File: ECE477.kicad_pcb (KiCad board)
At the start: 2 copper layers, 88.9 x 88.9 mm, 52 parts, among them IC1 LP3852EMP-3.3_NOPB, IC2 BQ29330DBT, J1 P7805-2000-S, J2 Conn_01x05_Male, J3 Conn_01x05_Male, J4 Conn_01x05_Male, J5 Conn_01x05_Male, J6 Conn_01x05_Male, J7 Conn_01x05_Male, J8 Conn_01x05_Male, SW1 SW_Push_Dual, U1 STM32H7_LQFP144_T2

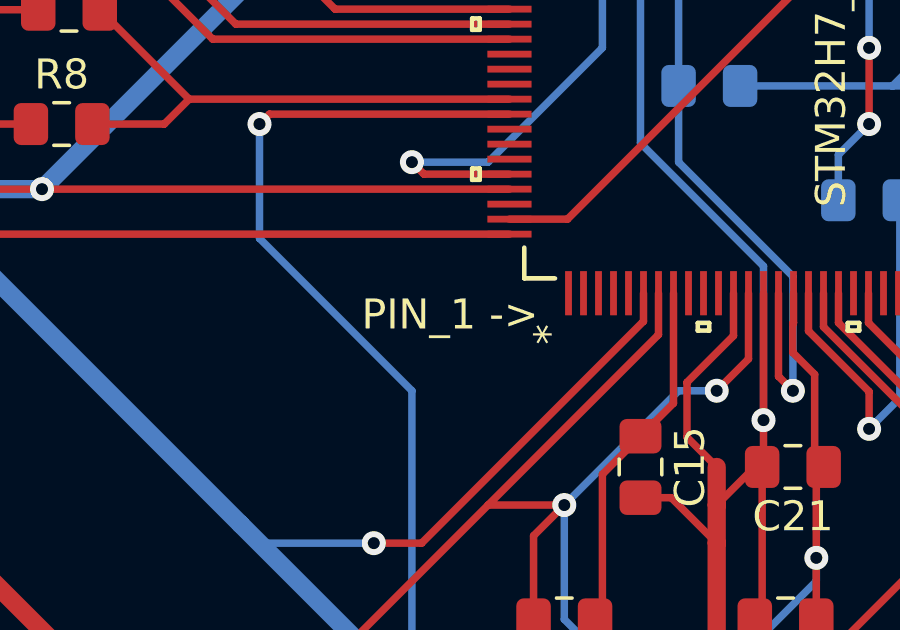
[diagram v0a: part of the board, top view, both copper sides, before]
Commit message: Updated
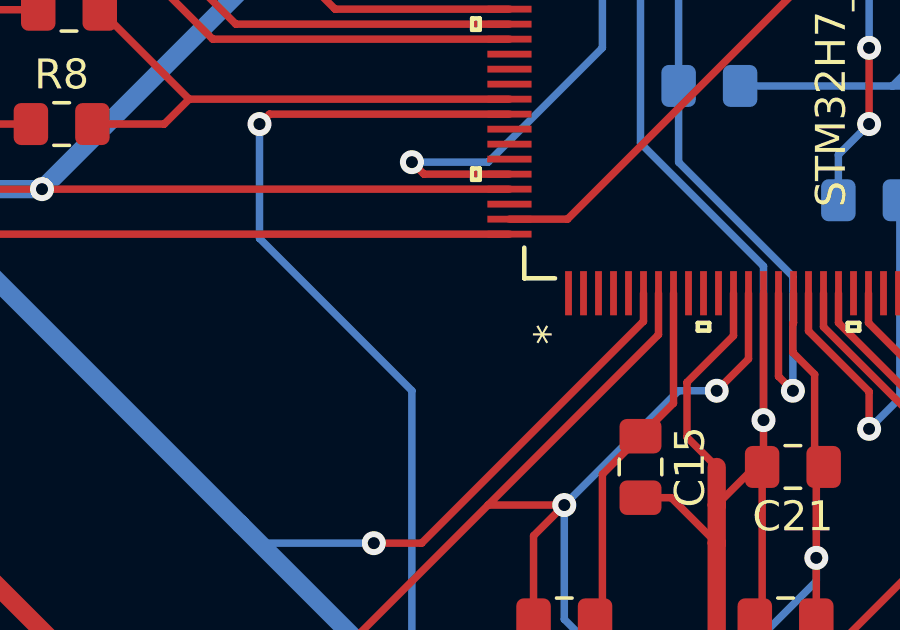
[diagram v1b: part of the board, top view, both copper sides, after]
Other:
- board text removed: "PIN_1 ->"
